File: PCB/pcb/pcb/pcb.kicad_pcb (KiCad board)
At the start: 2 copper layers, 69.6 x 60.2 mm, 28 parts

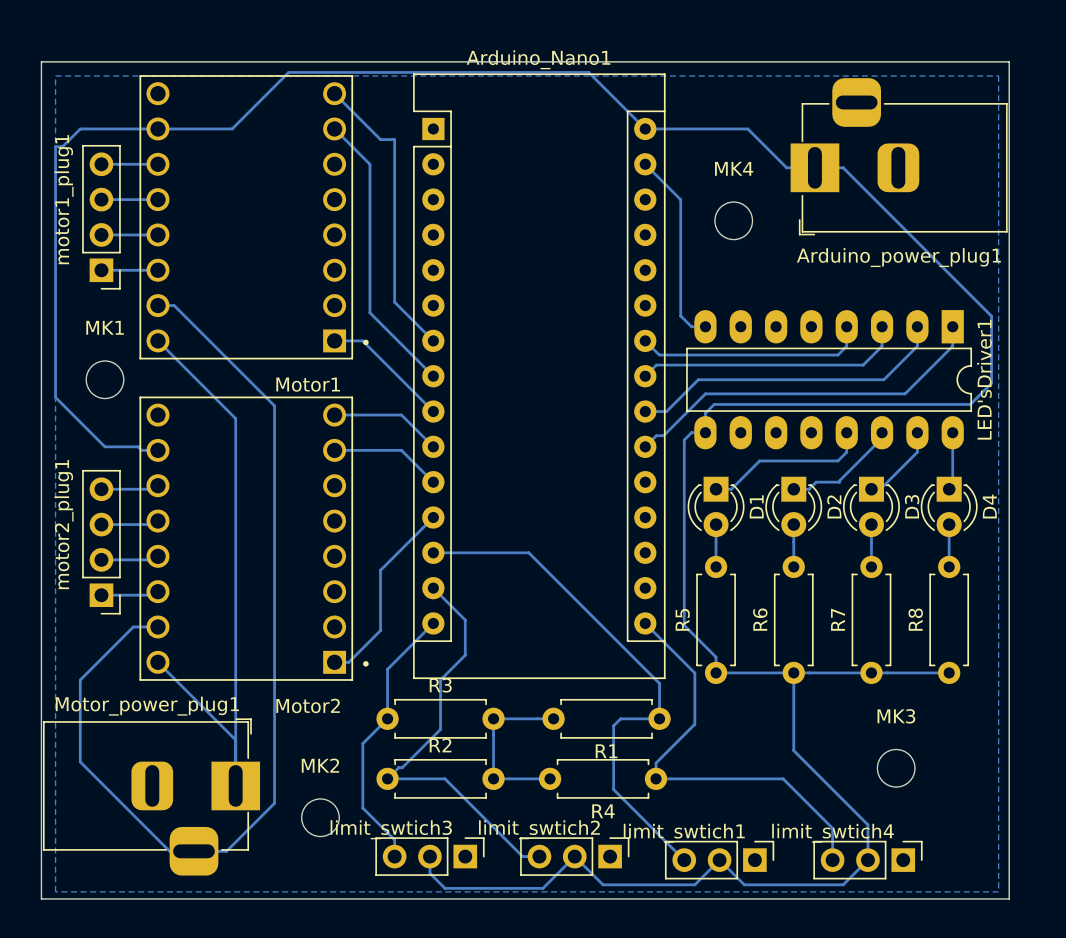
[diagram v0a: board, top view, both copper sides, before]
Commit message: V0.8 pcb Finished this closes #9 and closes #8
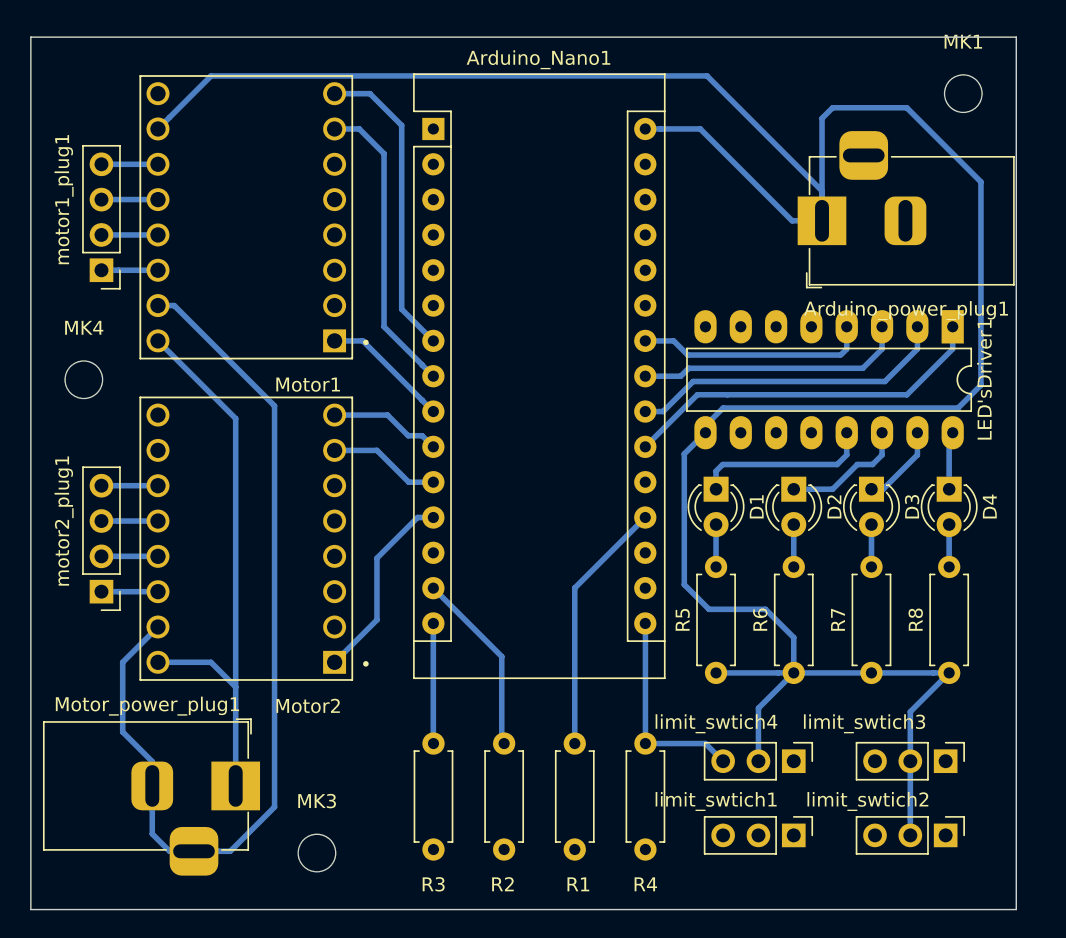
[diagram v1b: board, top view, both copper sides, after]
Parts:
- removed MK2: M2.5, MountingHole:MountingHole_2.7mm_M2.5
- moved MK1 65.1 mm to (244.2, 114.7)
- moved MK4 48.1 mm to (180.9, 135.3)
- moved MK3 42.1 mm to (197.7, 169.3)
- moved limit_swtich3 35.2 mm to (242.9, 162.7)
- moved limit_swtich2 24.2 mm to (242.9, 168.0)
- moved limit_swtich4 10.6 mm to (232.0, 162.7)
- moved R2 8.76 mm to (211.2, 161.4), turned to 270 degrees
- moved R1 6.35 mm to (216.3, 161.4), turned to 270 degrees
- moved Arduino_power_plug1 3.84 mm to (234.0, 123.8)
- moved R3 3.75 mm to (206.1, 161.4), turned to 270 degrees
- moved limit_swtich1 3.31 mm to (232.0, 168.0)
- moved R4 2.65 mm to (221.3, 161.4), turned to 270 degrees
- moved motor2_plug1 0.25 mm to (182.2, 150.5)
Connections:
- Arduino_Nano1 pad 13: Limit_switch4 -> Net-(Arduino_Nano1-Pad13)
- Arduino_Nano1 pad 14: Limit_switch3 -> Limit_switch2
- Arduino_Nano1 pad 15: Limit_switch2 -> Limit_switch3
- Arduino_Nano1 pad 16: Limit_switch1 -> Limit_switch4
- Arduino_Nano1 pad 19: Net-(Arduino_Nano1-Pad19) -> Limit_switch1
- Arduino_Nano1 pad 4: GND -> Net-(Arduino_Nano1-Pad4)
- Arduino_power_plug1 pad 2: Net-(Arduino_power_plug1-Pad2) -> GND
- Motor_power_plug1 pad 2: Net-(Motor_power_plug1-Pad2) -> GND_motor
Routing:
- net +5V: track 220.5 -> 188.4 mm
- net GND: track 26.8 -> 0.00 mm
- net Limit_switch1: track 38.0 -> 18.4 mm
- net Limit_switch2: track 30.4 -> 13.2 mm
- net Limit_switch4: track 30.3 -> 14.8 mm
- net Limit_switch3: track 19.8 -> 8.74 mm
- net Vmot_1: track 45.5 -> 40.6 mm
- net GND_motor: track 71.1 -> 67.7 mm
- net Step_motor1: track 20.7 -> 21.8 mm
- net Dir_motor1: track 21.3 -> 22.2 mm
- net S_LED1: track 11.9 -> 12.8 mm
- net S_LED2: track 8.33 -> 8.97 mm
- removed copper zone on B.Cu, net GND
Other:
- board size 69.6 x 60.2 mm -> 70.9 x 62.7 mm
- net class Default: clearance 0.2 -> 0.25; trace_width 0.2 -> 0.4
- net class Power: clearance 0.2 -> 0.25; trace_width 0.5 -> 0.4
- rule trace_clearance: 0.2 -> 0.25
- rule trace_min: 0.1524 -> 0.2
